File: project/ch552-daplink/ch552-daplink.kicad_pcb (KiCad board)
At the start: 2 copper layers, 22 x 11.5 mm, 21 parts, among them J1 USB_C_Receptacle_USB2.0_16P, J3 BOOT, U1 CH552E

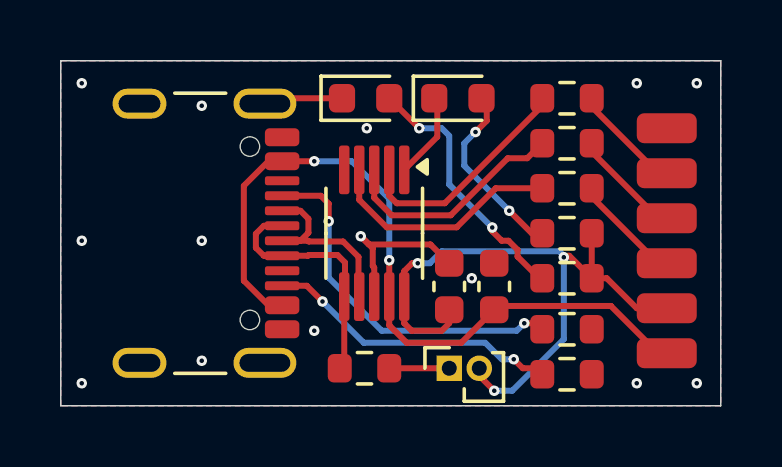
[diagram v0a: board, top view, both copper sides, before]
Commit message: 2025/07/21/19:40
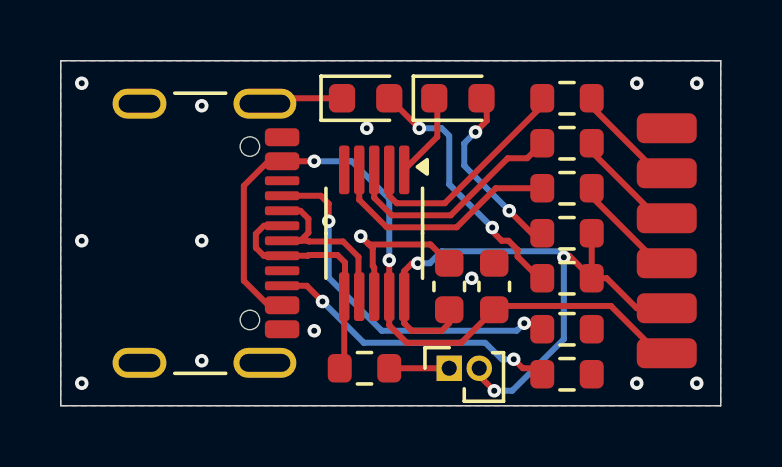
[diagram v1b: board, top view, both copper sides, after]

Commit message: 2025/07/21/20:12
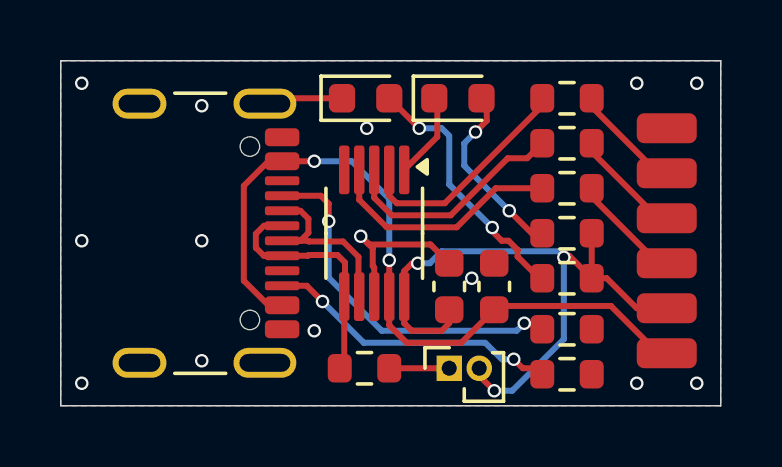
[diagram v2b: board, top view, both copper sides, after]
